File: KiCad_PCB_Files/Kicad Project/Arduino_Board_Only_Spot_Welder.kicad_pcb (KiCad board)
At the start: 2 copper layers, 110 x 60 mm, 71 parts, among them P1 MCP1407, P2 GND_con, P3 AutoPulse, P4 GND_con, P5 AutoPulse, P6 OLED_Display, Q1 IRFB_7430, Q2 IRFB_7430, Q3 IRFB_7430, Q4 IRFB_7430, Q5 IRFB_7430, Q6 IRFB_7430, Q7 IRFB_7430, Q8 IRFB_7430, U1 arduino_nano

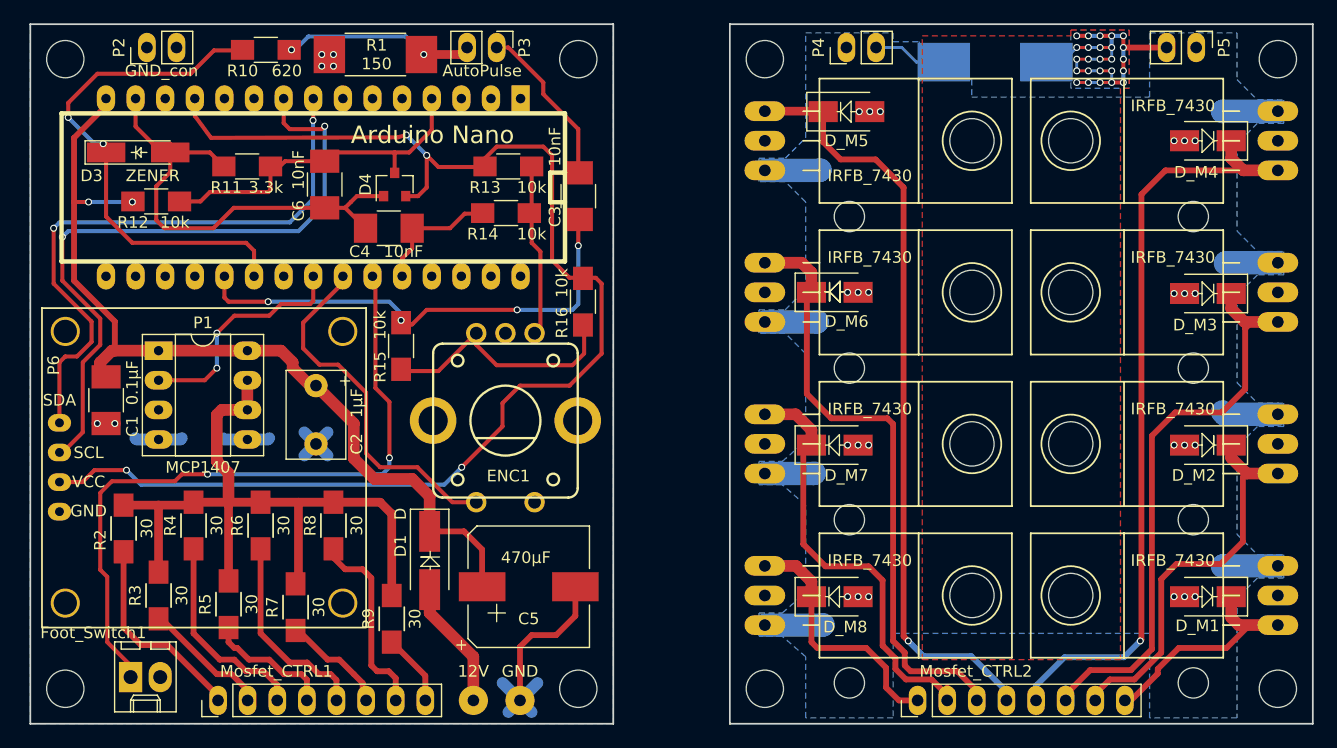
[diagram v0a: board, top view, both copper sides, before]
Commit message: Add files via upload
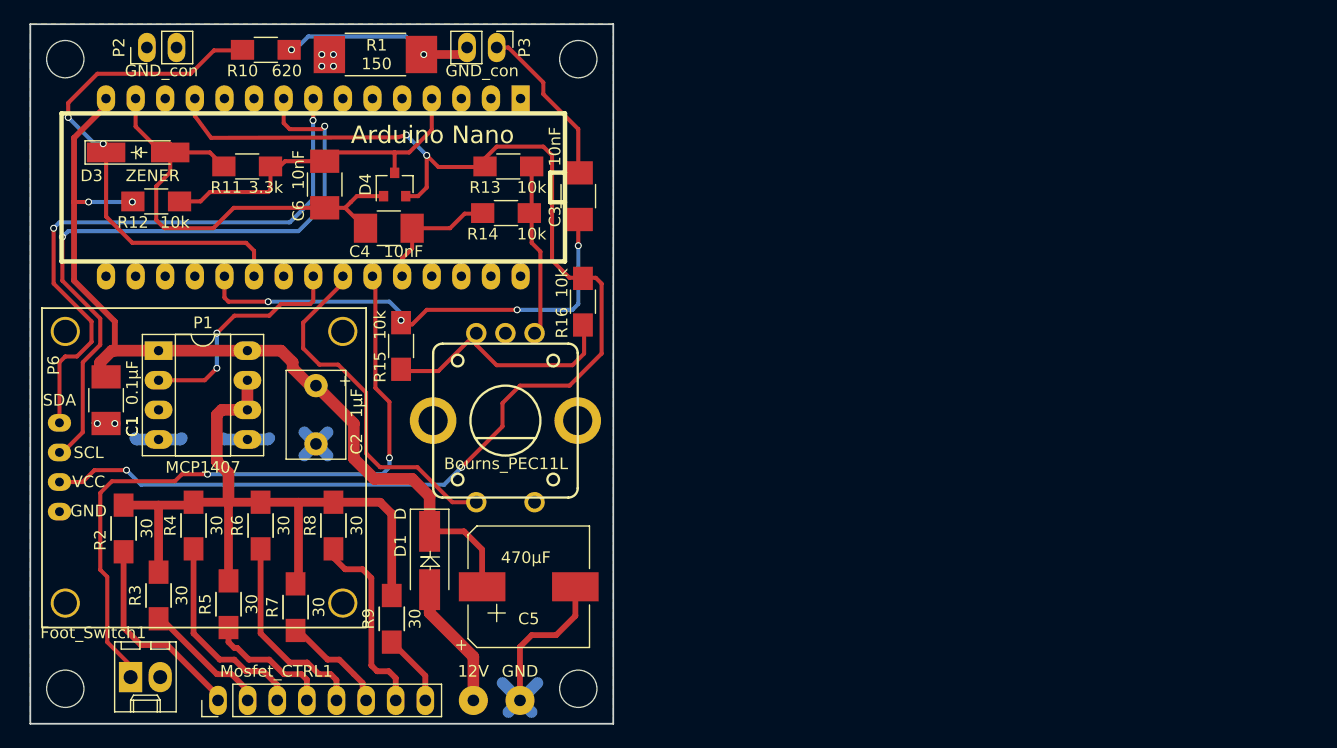
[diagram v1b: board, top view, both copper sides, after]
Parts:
- removed D_M1, D_M2, D_M3, D_M4, D_M5, D_M6, D_M7, D_M8: TVS-SMAJ13A-13-F, Diodes_SMD:D_SMA
- removed ENC1: Bourns_PEC11L, Rotary-Encoders:ALPS_STEC12E08
- removed Mosfet_CTRL2: CONN_01X08, pots_own:Pin_Header_Straight_1x08_Pitch2.54mm_Large_Pads
- removed P4: GND_con, Pin_Headers:Pin_Header_Straight_1x02_Pitch2.54mm
- removed P5: AutoPulse, Pin_Headers:Pin_Header_Straight_1x02_Pitch2.54mm
- removed Q1, Q2, Q3, Q4, Q5, Q6, Q7, Q8: IRFB_7430, pots_own:TO-220__long_Neutral123_Horizontal_LargePads
- removed the REF** at (169.8, 86.5)
- removed the REF** at (177.0, 73.0)
- removed the REF** at (133.0, 73.0)
- removed the REF** at (140.2, 86.5)
- removed the REF** at (169.8, 99.5)
- removed the REF** at (169.8, 112.5)
- removed the REF** at (169.8, 126.5)
- removed the REF** at (140.2, 126.5)
- removed the REF** at (140.2, 112.5)
- removed the REF** at (140.2, 99.5)
- removed the REF** at (133.0, 127.0)
- removed the REF** at (177.0, 127.0)
- removed TVS1: 5.0SMDJ13A, Diodes_SMD:D_SMC_Handsoldering
- added C1: Bourns_PEC11L, Rotary-Encoders:ALPS_STEC12E08, F.Cu at (110.8, 104.0)
- P3: value AutoPulse -> GND_con
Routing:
- net /battery_minus: track 76.6 -> 0.00 mm, vias 24 -> 0
- net Net-(D_M4-Pad1): track 69.1 -> 0.00 mm, vias 1 -> 0
- net Net-(D_M5-Pad1): track 67.3 -> 0.00 mm, vias 1 -> 0
- net Net-(D_M3-Pad1): track 54.6 -> 0.00 mm
- net Net-(D_M6-Pad1): track 53.0 -> 0.00 mm
- net Net-(D_M7-Pad1): track 38.9 -> 0.00 mm
- net Net-(D_M2-Pad1): track 37.7 -> 0.00 mm
- net /Probe: track 31.9 -> 0.00 mm, vias 25 -> 0
- net Net-(D_M1-Pad1): track 22.2 -> 0.00 mm
- net Net-(D_M8-Pad1): track 21.9 -> 0.00 mm
- removed copper zone on B.Cu, net /Probe
- removed copper zone on F.Cu, net /Probe
- removed copper zone on B.Cu, net /battery_minus
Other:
- board size 110 x 60 mm -> 50 x 60 mm
